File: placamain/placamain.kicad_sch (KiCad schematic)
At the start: 51 parts, among them J1 Conn_01x10_Pin, J2 Conn_01x10_Pin, Q1 PN3643, Q2 BC559, U1 LM393, U10 LF356, U2 LF356, U3 LF356, U4 LF356, U5 AD548JN, U6 LF356, U7 LF356, U8 LM393, U9 LM393

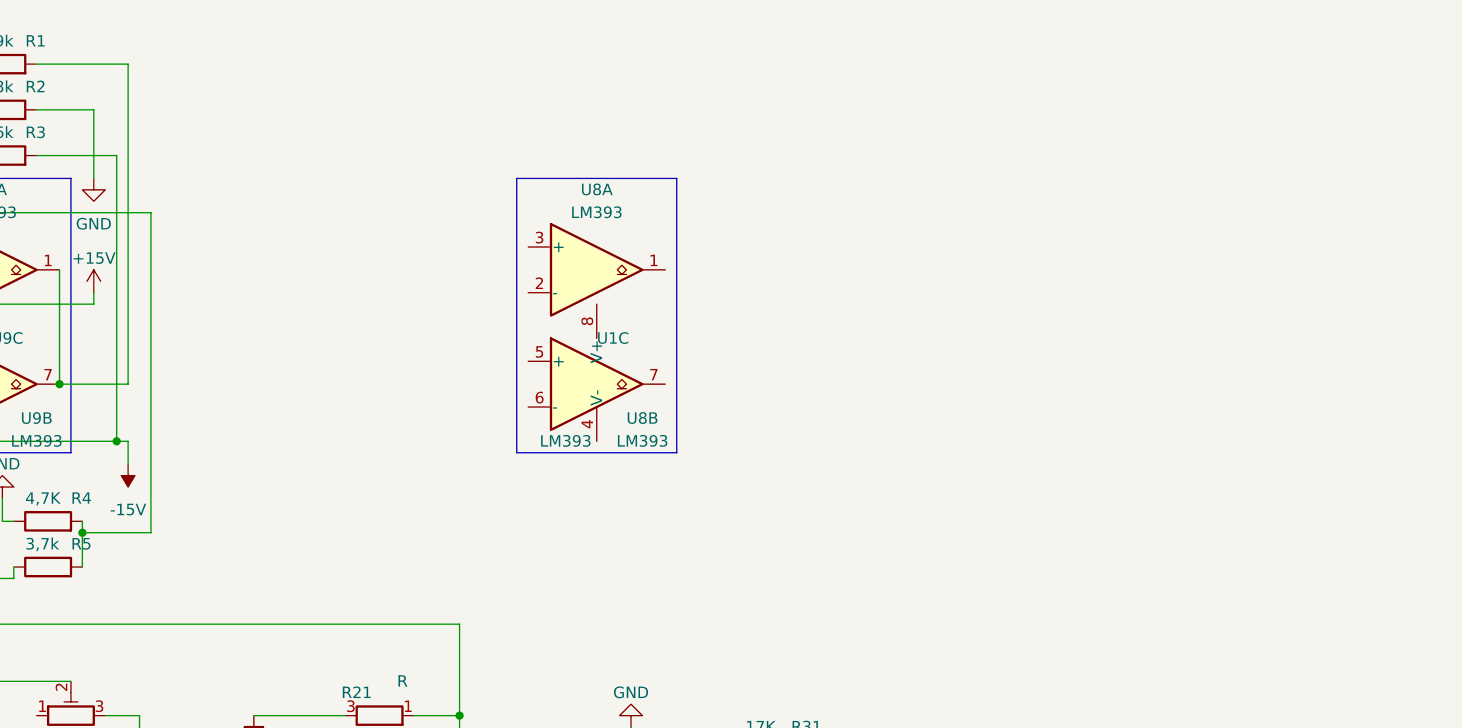
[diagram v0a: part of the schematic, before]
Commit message: Agrego CI12
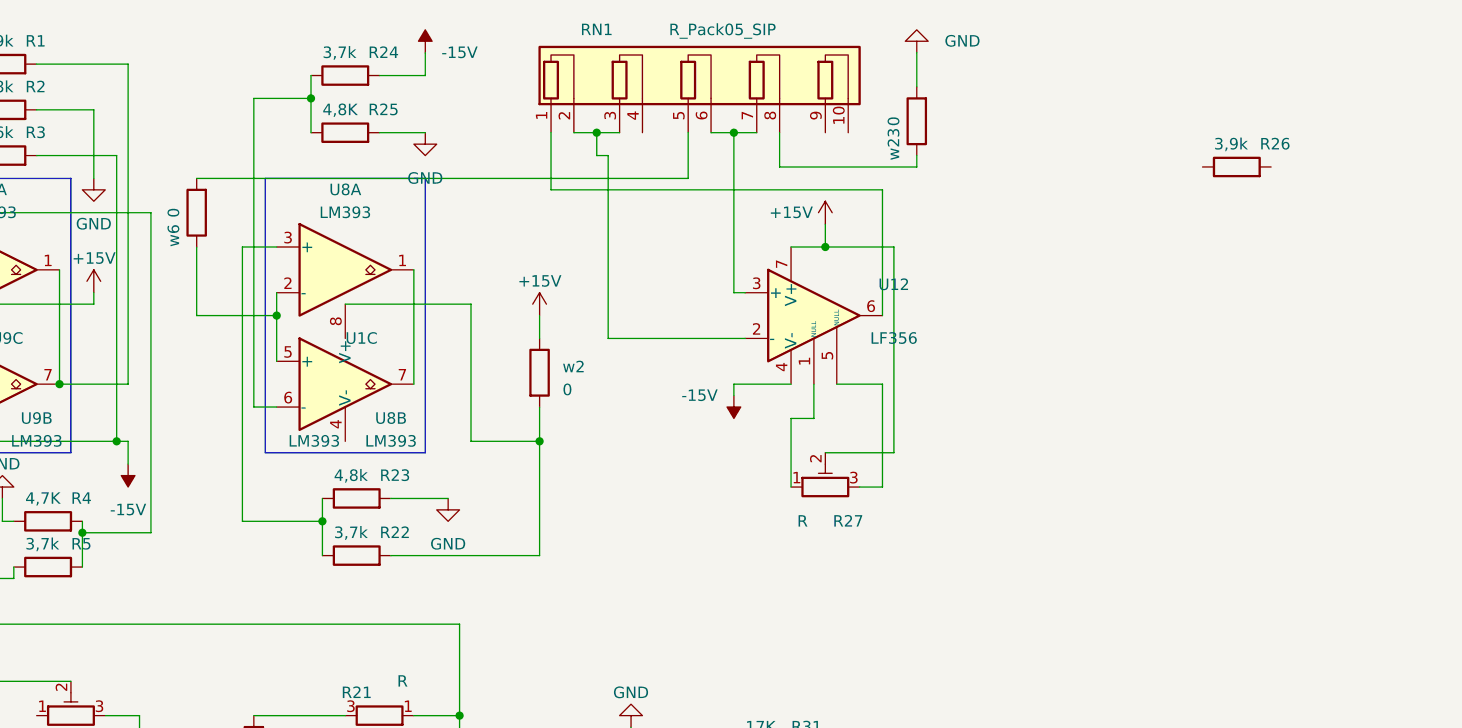
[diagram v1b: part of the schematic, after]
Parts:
- added R22, R24: 3,7k, symbol Device:R
- added R23: 4,8k, symbol Device:R
- added R25: 4,8K, symbol Device:R
- added R26: 3,9k, symbol Device:R
- added R27: R, symbol Device:R_Potentiometer_Trim
- added RN1: R_Pack05_SIP, Resistor_THT:R_Array_SIP10, symbol Device:R_Pack05_SIP
- added U12: LF356, symbol Amplifier_Operational:LF356
- added w2, w23, w6: 0, symbol Device:R
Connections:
- net +15V: now also R27.2, U12.7 (V+), w2.1
- net -15V: now also R24.2, U12.4 (V-)
- net GND: now also R23.2, R25.2, w23.2
- net at U8.5 (+): now also U8.2 (-), w6.1
- net at U8.6 (-): now also R24.1, R25.1
- net at U8.7: now also U8.1
- net at U8.3 (+): now also R22.1, R23.1
- net at U1.8 (V+): now also R22.2, w2.2
- new net: RN1.8 (R4.2), w23.1
- new net: RN1.5 (R3.1), w6.2
- new net: R27.1, U12.1 (NULL)
- new net: R27.3, U12.5 (NULL)
- new net: RN1.1 (R1.1), U12.6
- new net: RN1.2 (R1.2), RN1.3 (R2.1), U12.2 (-)
- new net: RN1.6 (R3.2), RN1.7 (R4.1), U12.3 (+)
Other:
- moved on the sheet: U1C, U8A, U8B
